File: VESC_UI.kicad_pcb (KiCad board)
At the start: 4 copper layers, 50 x 50 mm, 64 parts, among them J1 Hall_DRV5055-Q1, J2 Hall_DRV5055-Q1, J3 Conn_01x07_Male, J4 Conn_02x05_Female, J5 Conn_01x05_Male, J6 Conn_01x04_Male, J8 Conn_01x02_Male, J9 Conn_01x02_Male, Q1 Mosfet IRLML2060TRPBF, Q2 Mosfet IRLML2060TRPBF, SW1 Vertical push button, SW2 Vertical push button, SW3 Vertical push button, SW4 Vertical push button, SW5 Push button, U2 STM32F401CEU6, U3 M95M04-DR

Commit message: Merge display shield and update smd components case
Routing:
- added copper zone on In2.Cu, net +3V3
- added copper zone on In1.Cu, net GND
- removed copper zone on In2.Cu_+3.3, net +3V3
- removed copper zone on In1.Cu_GND, net GND
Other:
- net class Default removed
- net class bigPower removed
- net class power removed

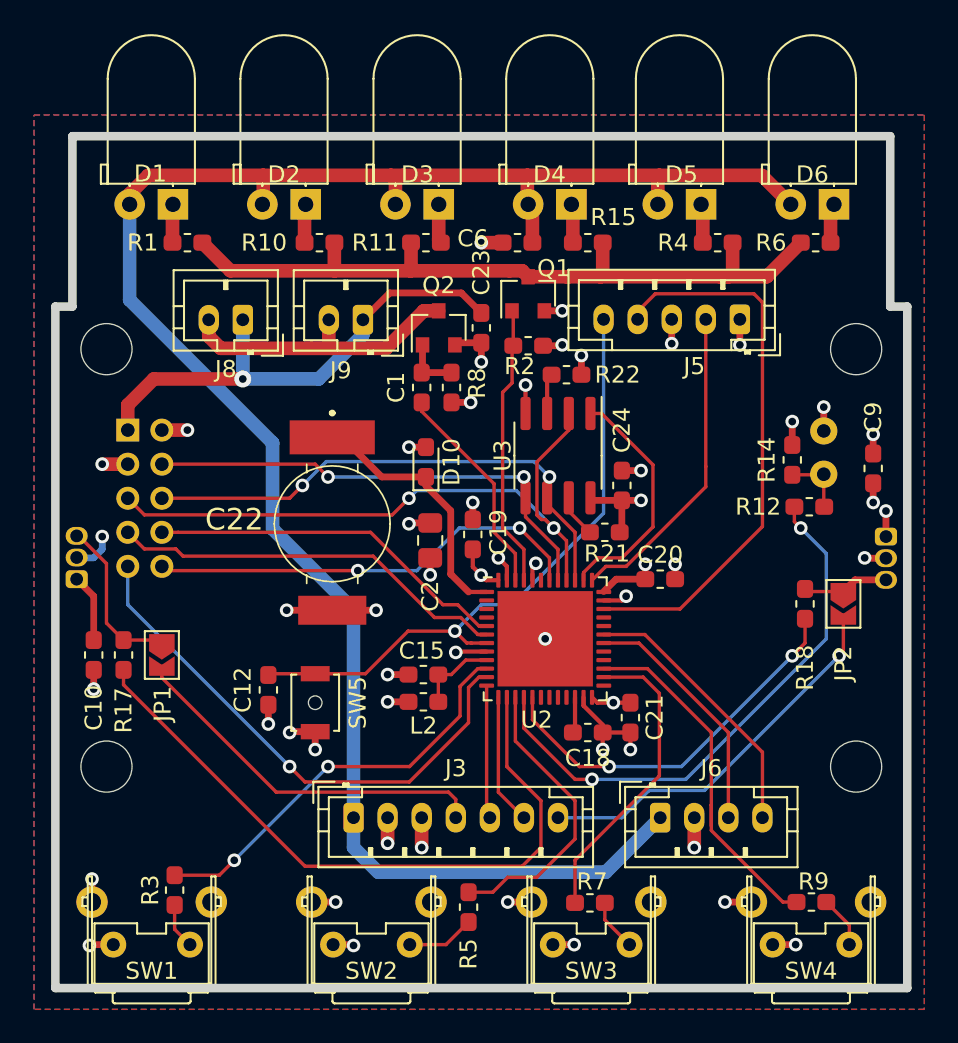
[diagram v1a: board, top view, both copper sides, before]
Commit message: Route complete
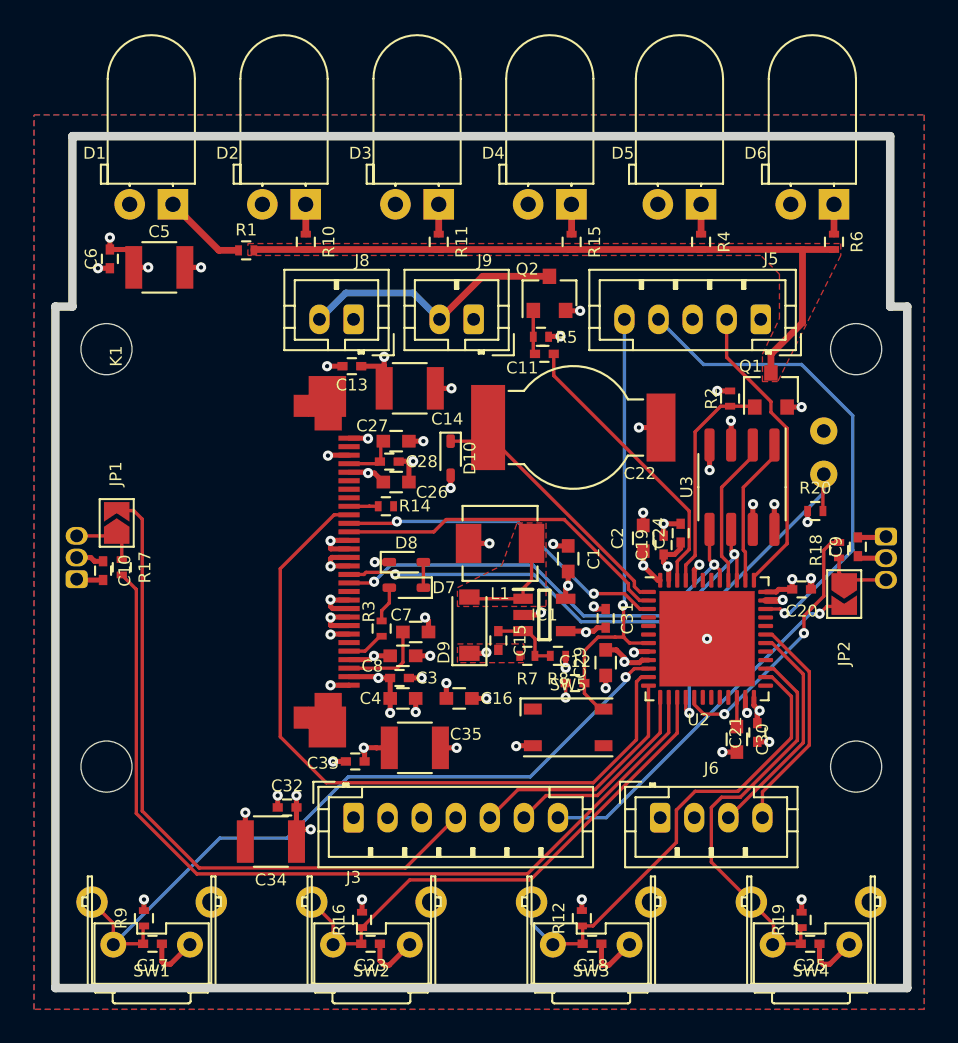
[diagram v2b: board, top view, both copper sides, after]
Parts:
- removed J4: Conn_02x05_Female, Connector_PinSocket_2.00mm:PinSocket_2x05_P2.00mm_Vertical
- removed L2: MMZ1608B121CTDH5, Inductor_SMD:L_0603_1608Metric_Pad1.05x0.95mm_HandSolder
- removed R21, R22: 10k, Resistor_SMD:R_0603_1608Metric_Pad1.05x0.95mm_HandSolder
- added C11: C_0002, DVB_Capacitors_Ceramic:C_0402, F.Cu at (142.7, 87.8)
- added C13: C_0002, DVB_Capacitors_Ceramic:C_0402, F.Cu at (131.4, 88.5)
- added C14: C_0040, DVB_Capacitors_Ceramic:C_1210, F.Cu at (134.8, 89.8)
- added C16: C_0003, DVB_Capacitors_Ceramic:C_0603, F.Cu at (137.7, 108.0)
- added C17: C_0002, DVB_Capacitors_Ceramic:C_0402, F.Cu at (119.7, 122.4)
- added C25: C_0002, DVB_Capacitors_Ceramic:C_0402, F.Cu at (158.3, 122.4)
- added C26: C_0037, DVB_Capacitors_Ceramic:C_0603, F.Cu at (134.0, 95.3)
- added C27: C_0003, DVB_Capacitors_Ceramic:C_0603, F.Cu at (134.0, 92.9)
- added C28: C_0002, DVB_Capacitors_Ceramic:C_0402, F.Cu at (133.6, 94.1)
- added C29: C_0037, DVB_Capacitors_Ceramic:C_0603, F.Cu at (146.3, 105.9)
- added C3: C_0002, DVB_Capacitors_Ceramic:C_0402, F.Cu at (134.2, 106.8)
- added C30: C_0003, DVB_Capacitors_Ceramic:C_0603, F.Cu at (154.0, 110.4)
- added C31: C_0002, DVB_Capacitors_Ceramic:C_0402, F.Cu at (146.3, 103.3)
- added C32: C_0002, DVB_Capacitors_Ceramic:C_0402, F.Cu at (127.6, 114.4)
- added C33: C_0002, DVB_Capacitors_Ceramic:C_0402, F.Cu at (131.6, 111.7)
- added C34: C_0040, DVB_Capacitors_Ceramic:C_1210, F.Cu at (126.7, 116.4)
- added C35: C_0040, DVB_Capacitors_Ceramic:C_1210, F.Cu at (135.1, 110.9)
- added C4: C_0003, DVB_Capacitors_Ceramic:C_0603, F.Cu at (134.4, 108.0)
- added C5: C_0040, DVB_Capacitors_Ceramic:C_1210, F.Cu at (120.1, 82.7)
- added C7: C_0003, DVB_Capacitors_Ceramic:C_0603, F.Cu at (135.2, 104.1)
- added C8: C_0037, DVB_Capacitors_Ceramic:C_0603, F.Cu at (134.4, 105.5)
- added D7: D_0022, DVB_Diodes:D_SOD-523-F, F.Cu at (134.6, 101.5)
- added D8: D_0022, DVB_Diodes:D_SOD-523-F, F.Cu at (134.6, 100.0)
- added D9: D_0016, DVB_Diodes:D_SOD-123, F.Cu at (138.3, 103.7)
- added IC1: FAN5331SX, SamacSys_Parts:SOT95P280X145-5N, F.Cu at (142.7, 103.1)
- added K1: K_0051-OBSOLETE, DVB_Displays:OLED128x128-1P5, B.Cu at (129.0, 100.0)
- added L1: L_0006, DVB_Inductors:L_4012-Wurth, F.Cu at (140.1, 98.9)
- added R16: R_0020, DVB_Resistors:R_0402, F.Cu at (132.0, 121.0)
- added R19: R_0020, DVB_Resistors:R_0402, F.Cu at (157.8, 121.0)
- added R20: R_0020, DVB_Resistors:R_0402, F.Cu at (158.6, 97.0)
- C1: value 10n -> C_0003; footprint Capacitor_SMD:C_0603_1608Metric_Pad1.05x0.95mm_HandSolder -> DVB_Capacitors_Ceramic:C_0603
- C10, C12, C19, C20, C21, C23, C24, C6, C9: value 100n -> C_0002; footprint Capacitor_SMD:C_0603_1608Metric_Pad1.05x0.95mm_HandSolder -> DVB_Capacitors_Ceramic:C_0402
- C15: value 100n -> C_0051; footprint Capacitor_SMD:C_0603_1608Metric_Pad1.05x0.95mm_HandSolder -> DVB_Capacitors_Ceramic:C_0402
- C18: value 4.7u -> C_0002; footprint Capacitor_SMD:C_0603_1608Metric_Pad1.05x0.95mm_HandSolder -> DVB_Capacitors_Ceramic:C_0402
- C2: value 10µF -> C_0003; footprint Capacitor_SMD:C_0805_2012Metric_Pad1.15x1.40mm_HandSolder -> DVB_Capacitors_Ceramic:C_0603
- C22: value SUpercap 330mF -> C_0046; footprint SamacSys_Parts:DSK3R3H334THL -> DVB_Capacitors_Supercap:CP_ELNA-DSK621
- D10: value Schottky CD0603-B0240R -> D_0022; footprint Diode_SMD:D_0603_1608Metric_Pad1.05x0.95mm_HandSolder -> DVB_Diodes:D_SOD-523-F
- Q1, Q2: value Mosfet IRLML2060TRPBF -> Q_0020; footprint Package_TO_SOT_SMD:SOT-23 -> DVB_SOT:SOT_23
- R1, R10, R11, R15, R4, R6: value 62 -> R_0110; footprint Resistor_SMD:R_0603_1608Metric_Pad1.05x0.95mm_HandSolder -> DVB_Resistors:R_0402
- R12, R9: value 100 -> R_0020; footprint Resistor_SMD:R_0603_1608Metric_Pad1.05x0.95mm_HandSolder -> DVB_Resistors:R_0402
- R14: value 10k -> R_0019; footprint Resistor_SMD:R_0603_1608Metric_Pad1.05x0.95mm_HandSolder -> DVB_Resistors:R_0402
- R17, R18: value 0 -> R_0001; footprint Resistor_SMD:R_0603_1608Metric_Pad1.05x0.95mm_HandSolder -> DVB_Resistors:R_0402
- R2: value 100k -> R_0034; footprint Resistor_SMD:R_0603_1608Metric_Pad1.05x0.95mm_HandSolder -> DVB_Resistors:R_0402
- R3: value 100 -> R_0110; footprint Resistor_SMD:R_0603_1608Metric_Pad1.05x0.95mm_HandSolder -> DVB_Resistors:R_0402
- R5, R7: value 100 -> R_0034; footprint Resistor_SMD:R_0603_1608Metric_Pad1.05x0.95mm_HandSolder -> DVB_Resistors:R_0402
- R8: value 1M -> R_0020; footprint Resistor_SMD:R_0603_1608Metric_Pad1.05x0.95mm_HandSolder -> DVB_Resistors:R_0402
- SW5: value Push button -> SW_0003; footprint Button_Switch_SMD:SW_SPST_B3U-1000P-B -> DVB_Buttons:PTS810
- U2: value STM32F401CEU6 -> STM32F401CEUx
- moved R9 39.2 mm to (119.2, 120.9), turned to 90 degrees
- moved C23 36.7 mm to (132.5, 122.4), turned to 180 degrees
- moved R5 33.7 mm to (142.5, 86.8), turned to 180 degrees
- moved R12 27.6 mm to (144.9, 120.9), turned to 90 degrees
- moved R14 24.0 mm to (133.4, 96.7), turned to 0 degrees
- moved C6 23.9 mm to (117.2, 82.2), turned to 90 degrees
- moved R3 19.6 mm to (133.2, 103.9)
- moved C12 18.0 mm to (144.5, 107.1), turned to 0 degrees
- moved R8 16.9 mm to (143.5, 105.5), turned to 180 degrees
- moved Q1 15.3 mm to (156.0, 89.9)
- moved C22 15.2 mm to (144.4, 92.1)
- moved R7 15.0 mm to (141.7, 105.5)
- moved SW5 14.9 mm to (144.1, 109.7), turned to 0 degrees
- moved C1 13.2 mm to (144.1, 99.8)
- moved C2 12.5 mm to (148.5, 98.6)
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- renumbered REF** to Hole1, REF** to Hole2, REF** to Hole3, REF** to Hole4
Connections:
- C1 pad 1: Net-(C1-Pad1) -> GND
- C1 pad 2: /BUZZER -> +3.3V
- C10 pad 1: +3V3 -> GND
- C10 pad 2: GND -> +3.3V
- C12 pad 1: /NRST -> GND
- C12 pad 2: GND -> /NRST
- C15 pad 1: /VREF+ -> Net-(C15-Pad1)
- C15 pad 2: GND -> +12V
- C18 pad 1: Net-(C18-Pad1) -> GND
- C18 pad 2: GND -> /BUTTON_3
- C19 pad 1: +3V3 -> GND
- C19 pad 2: GND -> +3.3V
- C2 pad 1: +3V3 -> +3.3V
- C20 pad 1: +3V3 -> GND
- C20 pad 2: GND -> +3.3V
- C21 pad 1: +3V3 -> GND
- C21 pad 2: GND -> +3.3V
- C23 pad 1: +12V -> GND
- C23 pad 2: GND -> /BUTTON_2
- C24 pad 1: +3V3 -> GND
- C24 pad 2: GND -> +3.3V
- C9 pad 1: +3V3 -> GND
- C9 pad 2: GND -> +3.3V
- D10 pad 2: +3V3 -> +3.3V
- J1 pad 1: +3V3 -> +3.3V
- J2 pad 1: +3V3 -> +3.3V
- J3 pad 2: +3V3 -> +3.3V
- J5 pad 1: +3V3 -> +3.3V
- Q2 pad 1: Net-(C1-Pad1) -> Net-(C11-Pad2)
- R12 pad 1: Net-(R12-Pad1) -> /BUTTON_3
- R12 pad 2: /PHOTO_RESISTOR -> +3.3V
- R13 pad 1: +3V3 -> +3.3V
- R13 pad 2: Net-(R12-Pad1) -> /PHOTO_RESISTOR
- R14 pad 1: Net-(R12-Pad1) -> Net-(K1-Pad22)
- R2 pad 1: /LIGHT_SW -> GND
- R2 pad 2: GND -> /LIGHT_SW
- R3 pad 1: Net-(R3-Pad1) -> Net-(K1-Pad5)
- R3 pad 2: /BUTTON_1 -> Net-(D7-Pad2)
- R5 pad 1: Net-(R5-Pad1) -> GND
- R5 pad 2: /BUTTON_2 -> Net-(C11-Pad2)
- R7 pad 1: Net-(R7-Pad1) -> Net-(C15-Pad1)
- R7 pad 2: /BUTTON_3 -> +12V
- R8 pad 1: Net-(C1-Pad1) -> GND
- R8 pad 2: GND -> Net-(C15-Pad1)
- R9 pad 1: Net-(R9-Pad1) -> /BUTTON_1
- R9 pad 2: /BUTTON_4 -> +3.3V
- SW1 pad 1: GND -> /BUTTON_1
- SW1 pad 2: Net-(R3-Pad1) -> GND
- SW2 pad 1: GND -> /BUTTON_2
- SW2 pad 2: Net-(R5-Pad1) -> GND
- SW3 pad 1: GND -> /BUTTON_3
- SW3 pad 2: Net-(R7-Pad1) -> GND
- SW4 pad 1: GND -> /BUTTON_4
- SW4 pad 2: Net-(R9-Pad1) -> GND
- SW5 pad 1: /NRST -> unconnected-(SW5-Pad1)
- SW5 pad 2: GND -> /NRST
- U2 pad 18: Net-(U2-Pad18) -> (no net)
- U2 pad 19: Net-(U2-Pad19) -> (no net)
- U2 pad 2: Net-(U2-Pad2) -> /OLED_CS
- U2 pad 20: Net-(U2-Pad20) -> (no net)
- U2 pad 21: Net-(U2-Pad21) -> (no net)
- U2 pad 22: Net-(C18-Pad1) -> Net-(C30-Pad1)
- U2 pad 24: +3V3 -> +3.3V
- U2 pad 25: Net-(U2-Pad25) -> (no net)
- U2 pad 28: Net-(U2-Pad28) -> (no net)
- U2 pad 29: Net-(U2-Pad29) -> (no net)
- U2 pad 3: Net-(U2-Pad3) -> /OLED_DC
- U2 pad 32: Net-(U2-Pad32) -> (no net)
- U2 pad 33: Net-(U2-Pad33) -> (no net)
- U2 pad 36: +3V3 -> +3.3V
- U2 pad 4: Net-(U2-Pad4) -> (no net)
- U2 pad 42: /SD_CS -> (no net)
- U2 pad 43: Net-(U2-Pad43) -> (no net)
- U2 pad 48: +3V3 -> +3.3V
- U2 pad 5: /OLED_CS -> (no net)
- U2 pad 6: /OLED_DC -> (no net)
- U2 pad 9: /VREF+ -> +3.3V
- U3 pad 3: Net-(R22-Pad1) -> +3.3V
- U3 pad 7: Net-(R21-Pad1) -> +3.3V
- U3 pad 8: +3V3 -> +3.3V
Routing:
- net GND: track 60.0 -> 360.5 mm, vias 40 -> 48
- net +3.3V: track 0.00 -> 228.5 mm, vias 0 -> 19
- net +3V3: track 30.1 -> 0.00 mm, vias 14 -> 0
- net /SPI1_MISO: track 38.3 -> 8.86 mm, vias 2 -> 0
- net /SD_CS: track 25.9 -> 0.00 mm, vias 2 -> 0
- net +12V: track 29.4 -> 49.3 mm, vias 1 -> 5
- net /BUTTON_1: track 24.4 -> 44.1 mm, vias 2 -> 1
- net /Accelerator: track 21.9 -> 39.8 mm
- net /BUTTON_2: track 17.3 -> 31.0 mm
- net /ADC1: track 39.9 -> 52.6 mm
- net /PHOTO_RESISTOR: track 32.7 -> 20.5 mm, vias 2 -> 1
- net /OLED_RST: track 31.4 -> 42.5 mm, vias 1 -> 0
- net /NRST: track 37.8 -> 26.9 mm
- net +5V: track 113.1 -> 102.5 mm, vias 0 -> 4
- net /BUTTON_3: track 18.0 -> 28.3 mm
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- added copper zone on F.Cu, net +12V
- added copper zone on In2.Cu, net +12V
- added copper zone on In2.Cu, net +3.3V
- added copper zone on In2.Cu, net +5V
- added copper zone on F.Cu, net Net-(D9-Pad2)
- added copper zone on F.Cu, net Net-(Q1-Pad3)
- removed copper zone on In2.Cu, net +3V3
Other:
- board text added: "VESC_UI v2.0.0"

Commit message: v2.0.0 version
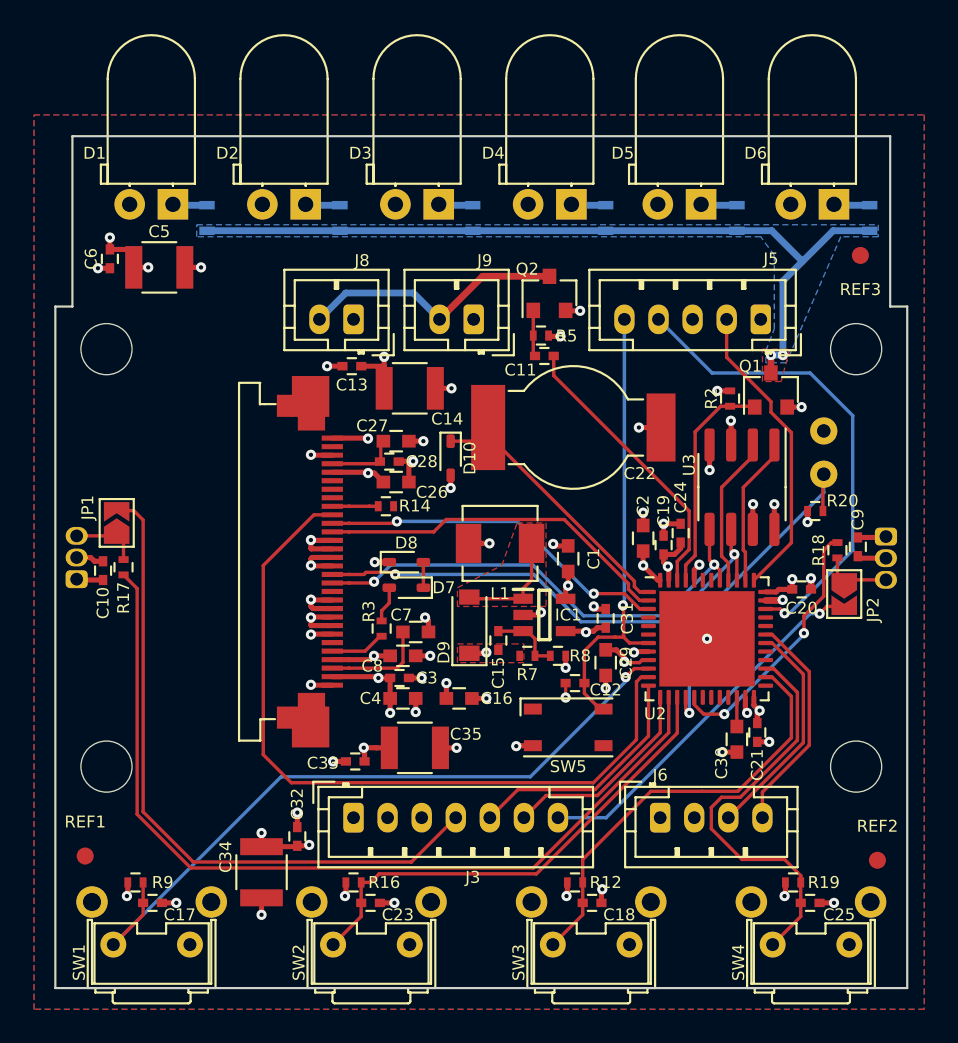
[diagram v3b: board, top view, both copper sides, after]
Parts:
- added REF1: CircleWhite1mm, DVB_Fiducials:REF_1mm, F.Cu at (115.8, 117.2)
- added REF2: CircleWhite1mm, DVB_Fiducials:REF_1mm, F.Cu at (162.2, 117.5)
- added REF3: CircleWhite1mm, DVB_Fiducials:REF_1mm, F.Cu at (161.2, 82.0)
- R1, R10, R11, R15, R4, R6: footprint DVB_Resistors:R_0402 -> DVB_Resistors:R_0603; moved to B.Cu
- SW1, SW2, SW3, SW4: footprint SamacSys_Parts:Vertical_push_button -> DVB_Buttons:Vertical_push_button
- moved K1 3.42 mm to (125.6, 100.0)
- moved R1 2.98 mm to (122.9, 79.8), turned to -90 degrees
- moved R6 2.52 mm to (161.8, 79.8)
- moved R4 2.52 mm to (154.0, 79.8)
- moved R10 2.44 mm to (130.7, 79.8)
- moved R11 2.44 mm to (138.5, 79.8)
- moved R15 2.44 mm to (146.3, 79.8)
- moved C17 2.40 mm to (119.7, 120.0)
- moved C18 2.40 mm to (145.5, 120.0)
- moved C23 2.40 mm to (132.5, 120.0)
- moved C25 2.40 mm to (158.3, 120.0)
- moved R16 2.26 mm to (131.5, 118.8), turned to 180 degrees
- moved R19 2.26 mm to (157.3, 118.8), turned to 180 degrees
- moved R9 2.16 mm to (118.7, 118.8), turned to 180 degrees
- moved R12 2.14 mm to (144.5, 118.8), turned to 180 degrees
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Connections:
- SW5 pad 1: unconnected-(SW5-Pad1) -> (no net)
- SW5 pad 4: unconnected-(SW5-Pad4) -> (no net)
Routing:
- net GND: track 360.5 -> 369.1 mm, vias 48 -> 52
- net Net-(Q1-Pad3): track 42.1 -> 48.1 mm, vias 0 -> 2
- net Net-(D1-Pad1): track 4.97 -> 2.02 mm
- net /BUTTON_3: track 28.3 -> 25.3 mm
- net +5V: track 102.5 -> 104.9 mm
- net /BUTTON_2: track 31.0 -> 28.6 mm
- net /OLED_RST: track 42.5 -> 44.2 mm
- net +3.3V: track 228.5 -> 230.1 mm
- net /BUTTON_1: track 44.1 -> 42.6 mm
- net Net-(C27-Pad1): track 3.15 -> 4.13 mm
- net Net-(K1-Pad5): track 2.27 -> 3.26 mm
- net +12V: track 49.3 -> 50.2 mm
- net /OLED_DC: track 19.8 -> 20.7 mm
- net /OLED_CS: track 20.0 -> 21.0 mm
- net Net-(K1-Pad22): track 1.71 -> 2.70 mm
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- added copper zone on B.Cu, net Net-(Q1-Pad3)

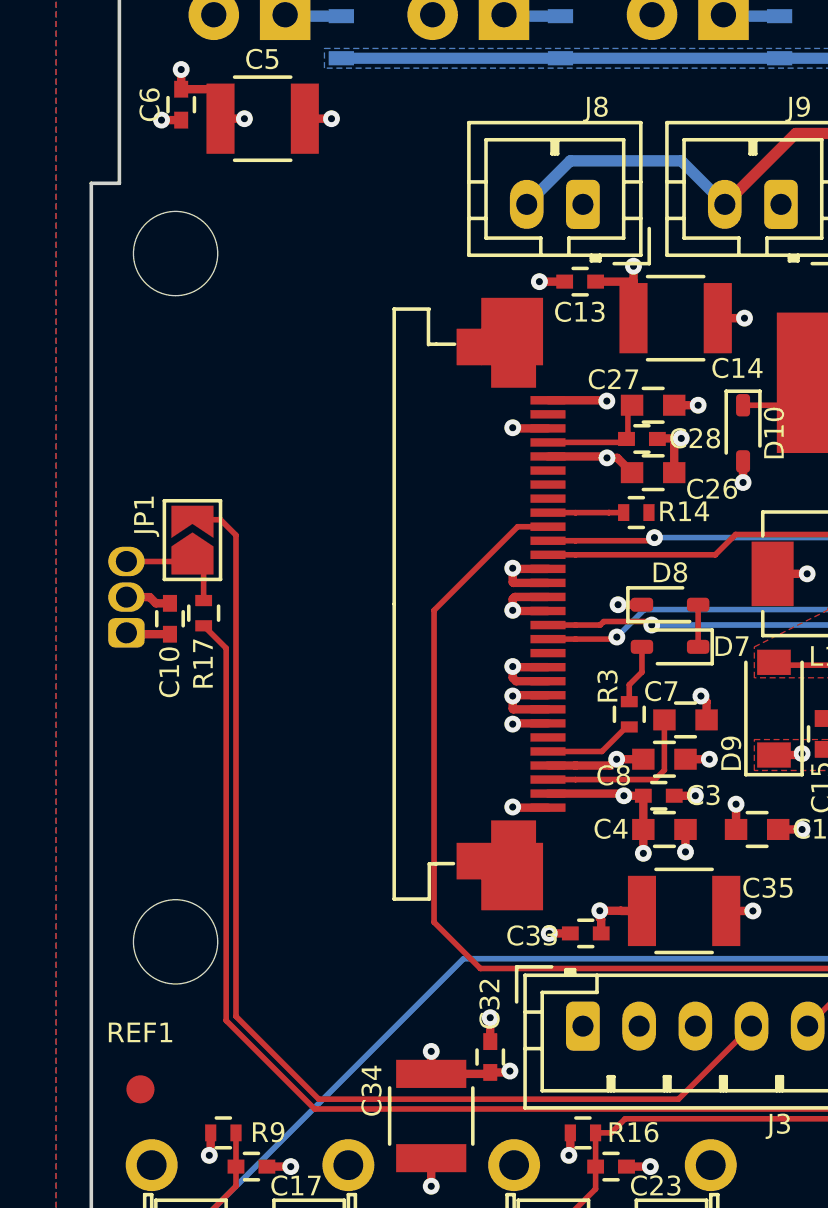
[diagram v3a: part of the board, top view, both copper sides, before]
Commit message: Update pos files
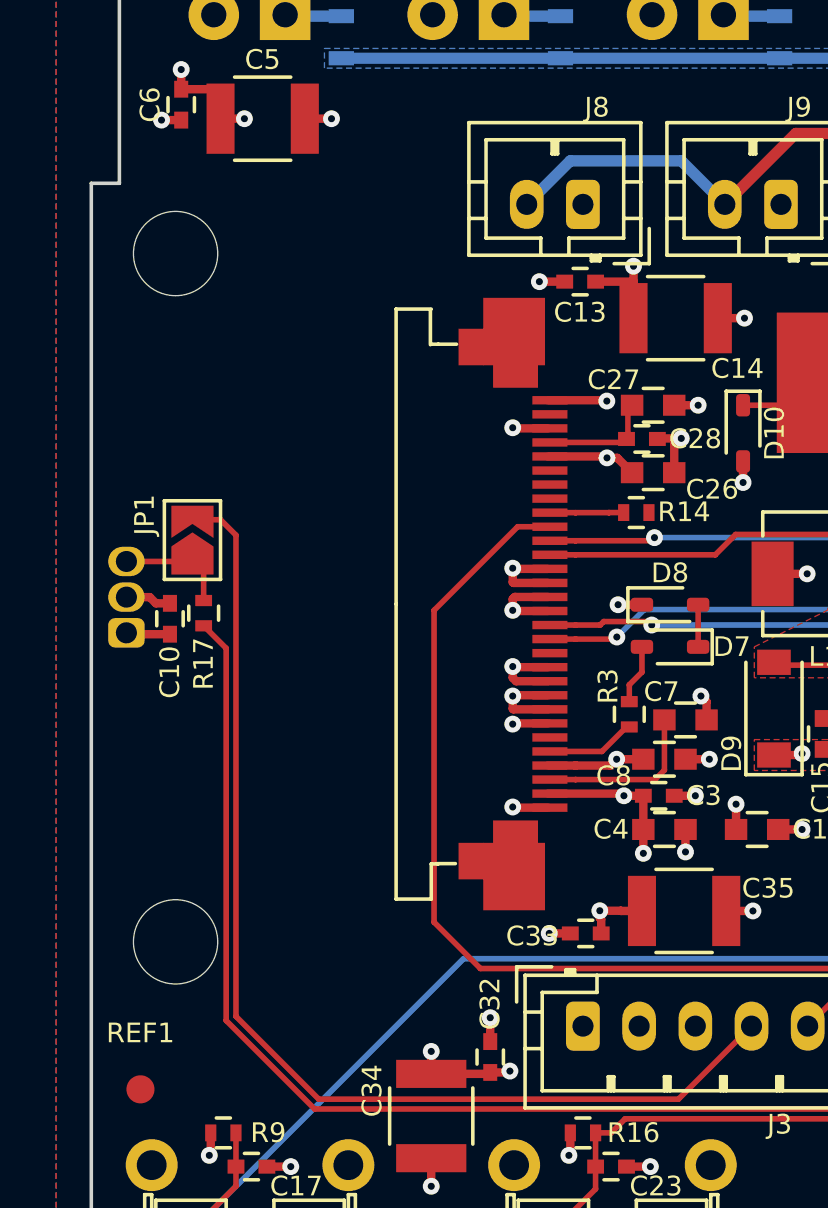
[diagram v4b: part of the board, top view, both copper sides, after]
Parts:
- K1: moved to F.Cu
- moved K1 1.42 mm to (127.0, 100.0), turned to -90 degrees
